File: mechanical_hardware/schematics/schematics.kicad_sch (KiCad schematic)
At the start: 19 parts, among them J1 Raspberry_Pi_4, J2 Encoder, J3 Encoder, M1 Motor_DC, M2 Motor_DC, SW1 PWR, U1 5.1V - Pi, U2 5V ESP32, U3 11.5V motors, U4 ESP32-C3, U5 MPU-9250

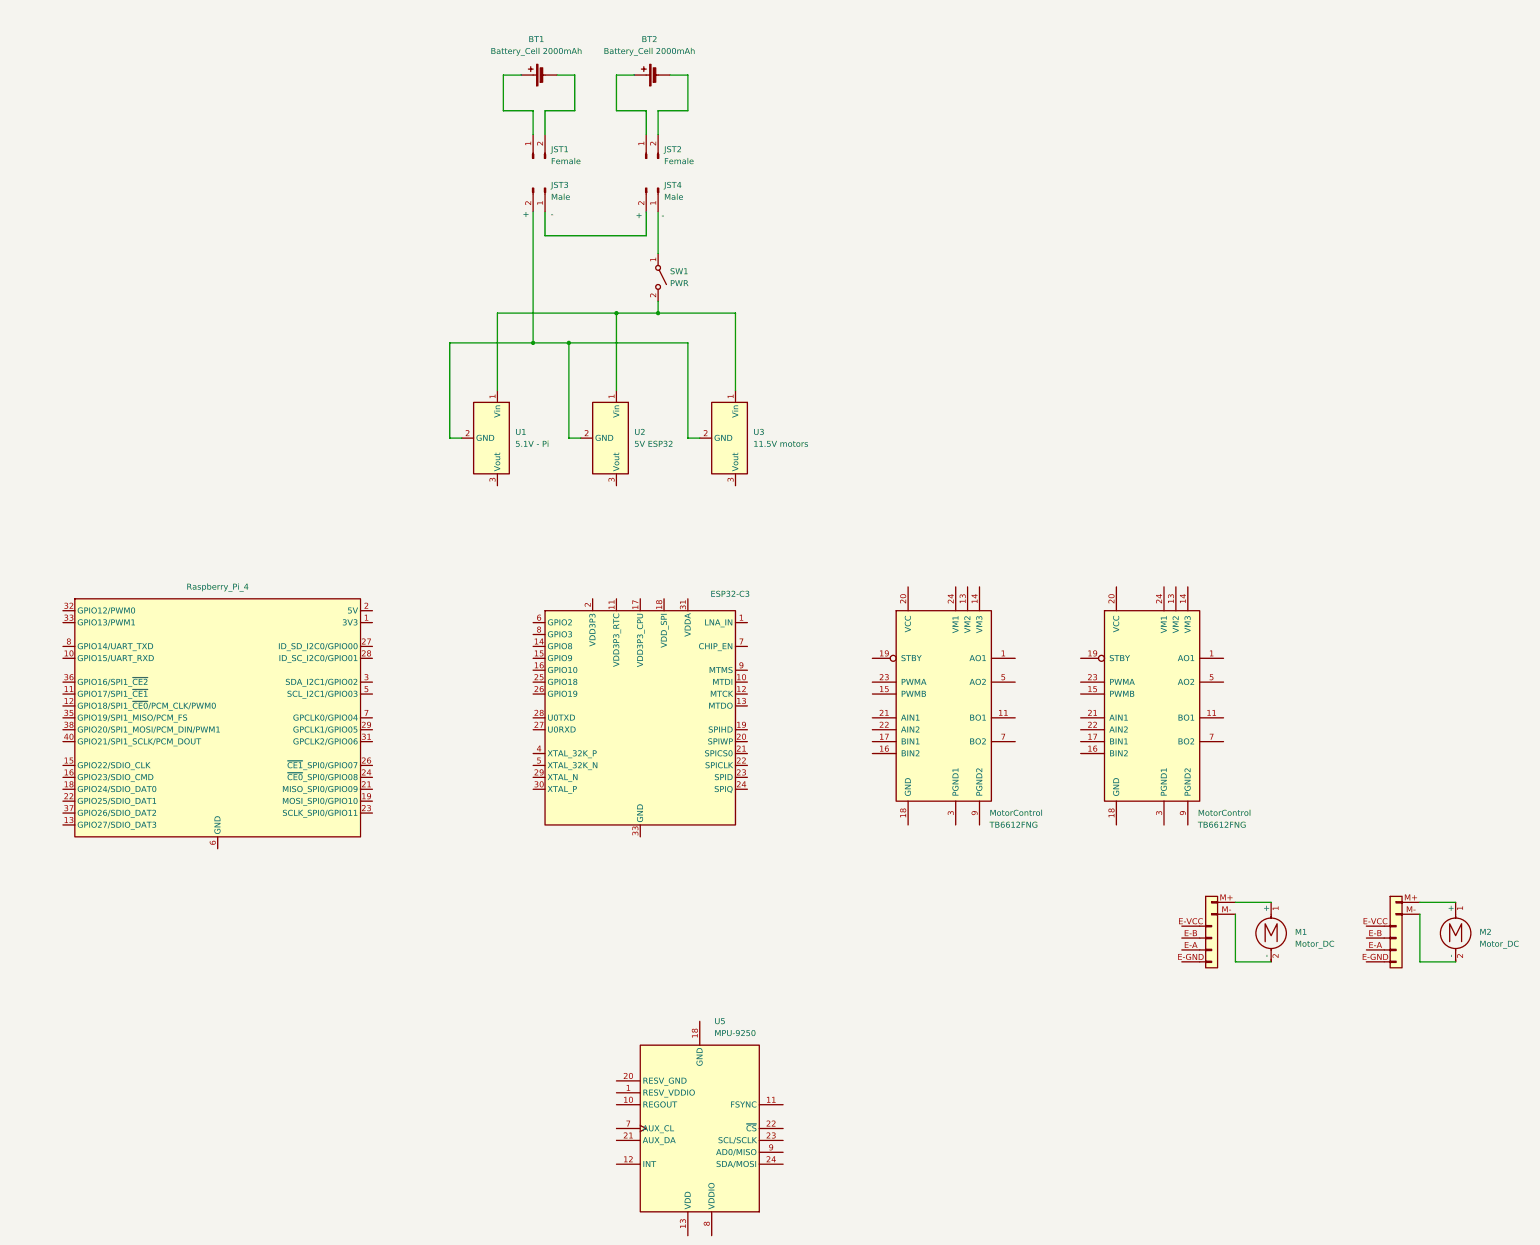
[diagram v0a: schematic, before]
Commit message: schematics
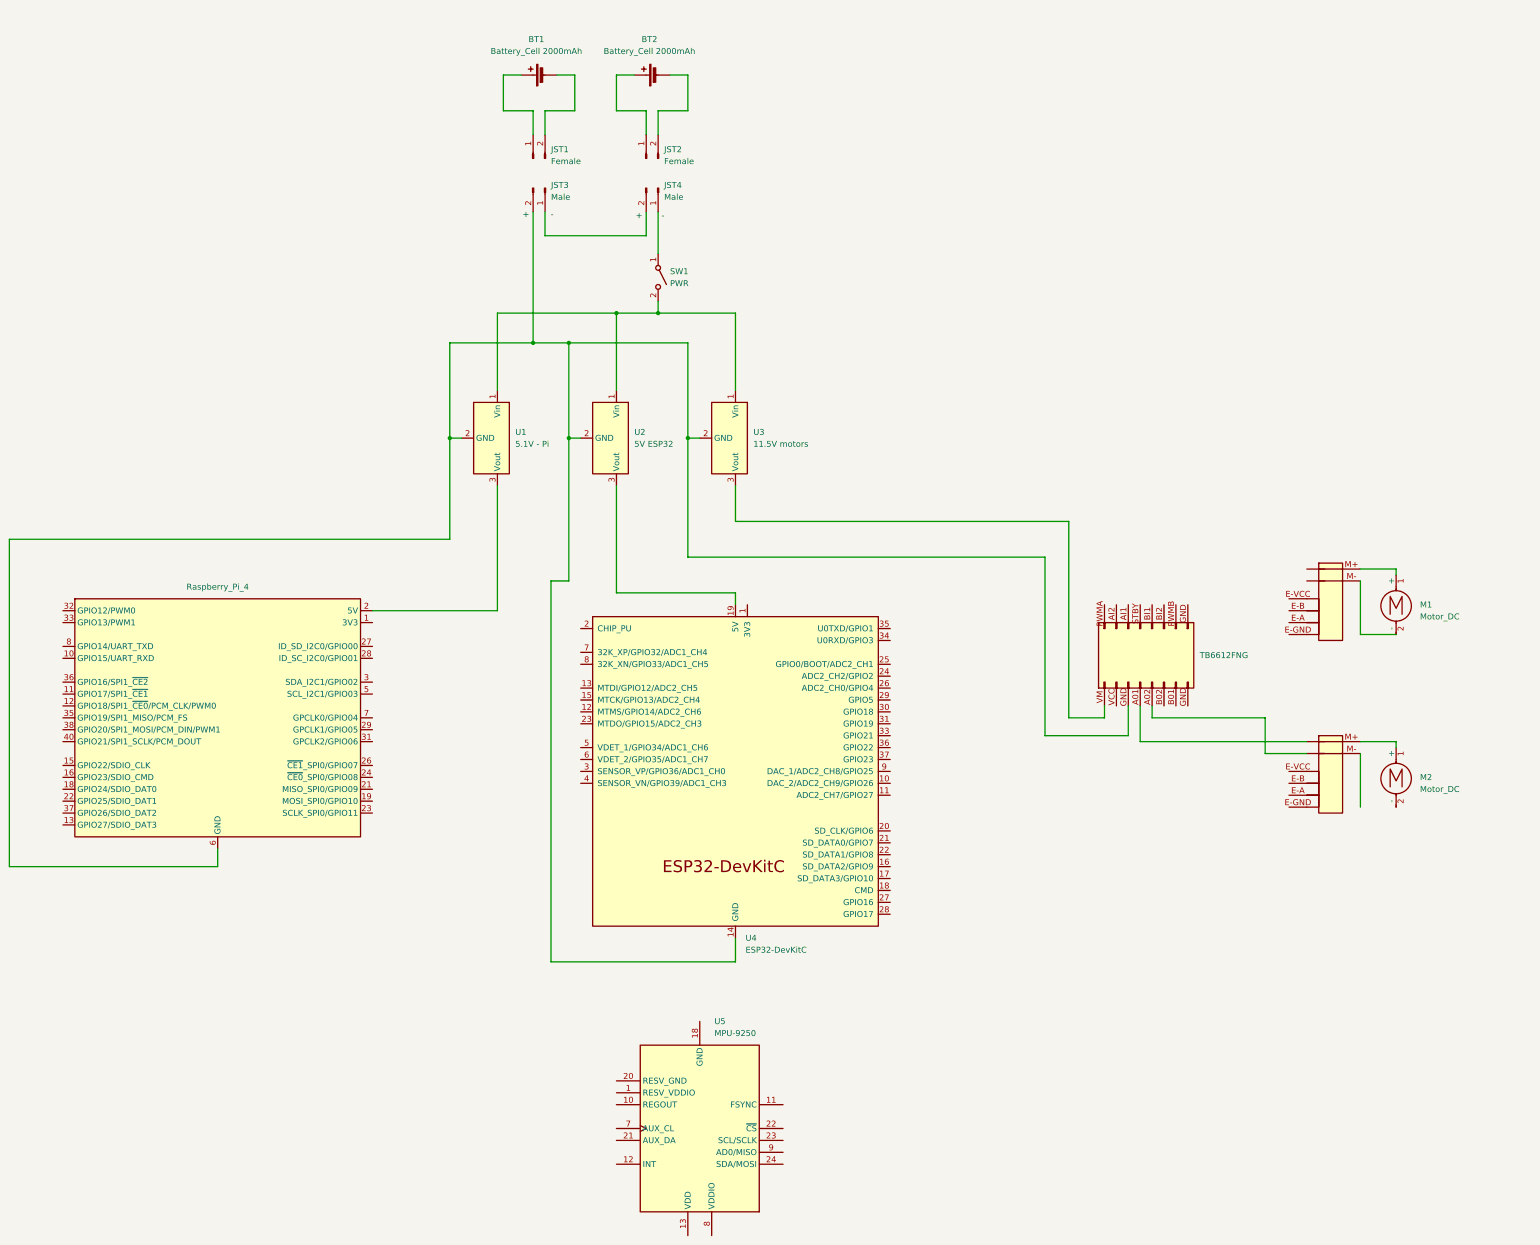
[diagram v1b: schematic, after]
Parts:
- removed J2, J3: Encoder, symbol Connector_Generic:Conn_01x06
- removed MotorControl (x2): TB6612FNG, Package_SO:SSOP-24_5.3x8.2mm_P0.65mm, symbol Driver_Motor:TB6612FNG
- removed U4: ESP32-C3, Package_DFN_QFN:QFN-32-1EP_5x5mm_P0.5mm_EP3.7x3.7mm, symbol MCU_Espressif:ESP32-C3
- added J4: TB6612FNG, symbol Connector_Generic:Conn_02x08_Top_Bottom
- added J5, J6: Encoder, symbol Connector_Generic:Conn_01x06
- added U4: ESP32-DevKitC, PCM_Espressif:ESP32-DevKitC, symbol PCM_Espressif:ESP32-DevKitC
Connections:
- net at M2.1 (+): now also J6.M+
- net at JST3.2 (Pin_2), U1.2 (GND), U2.2 (GND)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: now also J1.14 (GND), J1.20 (GND), J1.25 (GND), J1.30 (GND), J1.34 (GND), J1.39 (GND), J1.6 (GND), J1.9 (GND), J4.GND (Pin_16), U4.14 (GND), U4.32 (GND), U4.38 (GND)
- net at U1.3 (Vout): now also J1.2 (5V), J1.4 (5V)
- net at M1.1 (+): now also J5.M+
- net at M1.2 (-): now also J5.M-
- net at U2.3 (Vout): now also U4.19 (5V)
- net at U3.3 (Vout): now also J4.VM
- new net: J4.A01 (Pin_4), J6.
- new net: J4.A02 (Pin_5), J6.
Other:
- moved on the sheet: M1

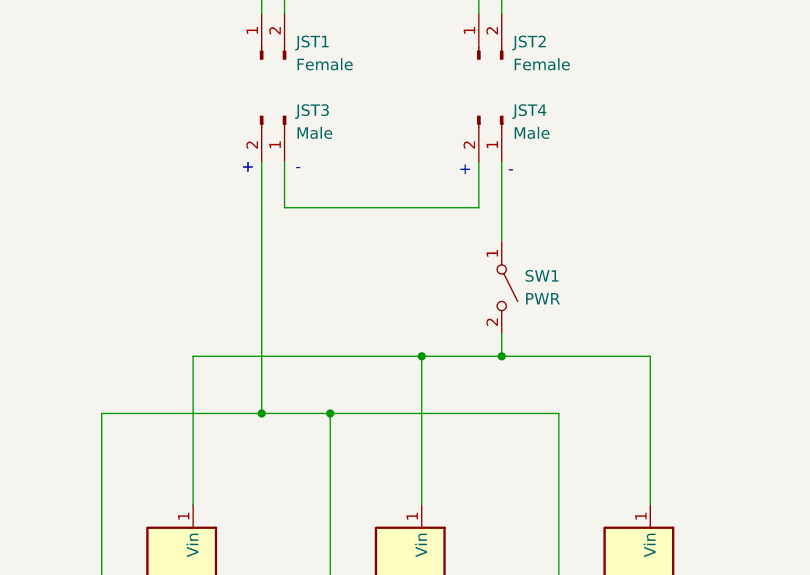
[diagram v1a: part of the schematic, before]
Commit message: fixed schematics
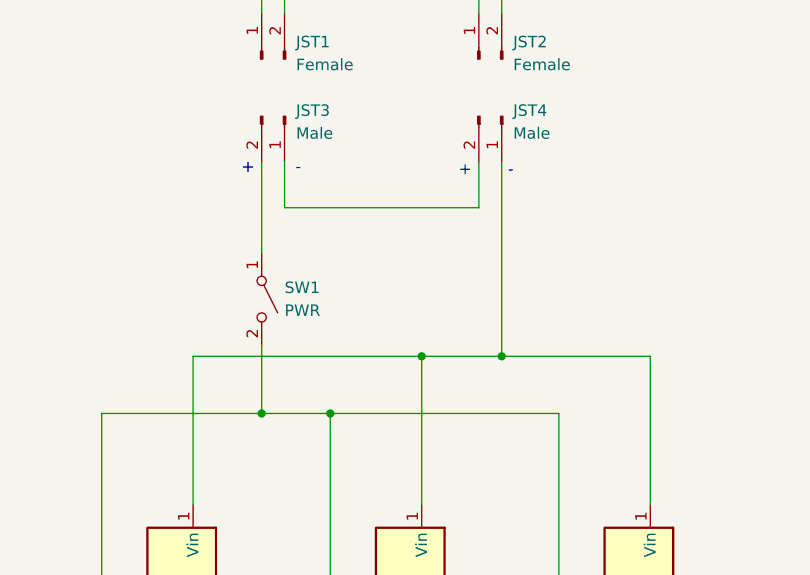
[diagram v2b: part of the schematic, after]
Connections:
- net at J4.GND (Pin_16): now also J1.14 (GND), J1.20 (GND), J1.25 (GND), J1.30 (GND), J1.34 (GND), J1.39 (GND), J1.6 (GND), J1.9 (GND), SW1.2 (B), U1.2 (GND), U2.2 (GND), U3.2 (GND), U4.14 (GND), U4.32 (GND), U4.38 (GND)
- net at SW1.1 (A): now also JST3.2 (Pin_2); no longer JST4.1 (Pin_1)
- net at U1.1 (Vin), U2.1 (Vin), U3.1 (Vin): now also JST4.1 (Pin_1); no longer SW1.2 (B)
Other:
- moved on the sheet: SW1
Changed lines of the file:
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@@
 	(wire
 		(pts
-			(xy 160.02 57.15) (xy 160.02 85.09)
+			(xy 160.02 57.15) (xy 160.02 67.31)
 		)
 		(stroke
@@
 	(wire
 		(pts
+			(xy 160.02 77.47) (xy 160.02 85.09)
+		)
+		(stroke
+			(width 0)
+			(type default)
+		)
+	)
+	(wire
+		(pts
 			(xy 336.55 170.18) (xy 344.17 170.18)
 		)
@@
 	(wire
 		(pts
-			(xy 186.69 76.2) (xy 186.69 78.74)
-		)
-		(stroke
-			(width 0)
-			(type default)
-		)
-	)
-	(wire
-		(pts
 			(xy 184.15 62.23) (xy 184.15 57.15)
 		)
@@
 	(wire
 		(pts
+			(xy 186.69 78.74) (xy 203.2 78.74)
+		)
+		(stroke
+			(width 0)
+			(type default)
+		)
+	)
+	(wire
+		(pts
 			(xy 316.23 165.1) (xy 316.23 172.72)
 		)
@@
 	(wire
 		(pts
+			(xy 186.69 57.15) (xy 186.69 78.74)
+		)
+		(stroke
+			(width 0)
+			(type default)
+		)
+	)
+	(wire
+		(pts
 			(xy 163.83 135.89) (xy 163.83 217.17)
 		)
@@
 	(wire
 		(pts
-			(xy 186.69 78.74) (xy 203.2 78.74)
-		)
-		(stroke
-			(width 0)
-			(type default)
-		)
-	)
-	(wire
-		(pts
 			(xy 153.67 27.94) (xy 153.67 35.56)
 		)
@@
 		(pts
 			(xy 186.69 35.56) (xy 186.69 40.64)
-		)
-		(stroke
-			(width 0)
-			(type default)
-		)
-	)
-	(wire
-		(pts
-			(xy 186.69 57.15) (xy 186.69 66.04)
 		)
 		(stroke
@@
 	(symbol
 		(lib_id "Switch:SW_SPST")
-		(at 186.69 71.12 270)
+		(at 160.02 72.39 270)
 		(unit 1)
 		(body_style 1)
@@
 		(fields_autoplaced yes)
 		(property "Reference" "SW1"
-			(at 189.23 69.8499 90)
+			(at 162.56 71.1199 90)
 			(show_name no)
 			(do_not_autoplace no)
@@
 		)
 		(property "Value" "PWR"
-			(at 189.23 72.3899 90)
+			(at 162.56 73.6599 90)
 			(show_name no)
 			(do_not_autoplace no)
@@
 		)
 		(property "Footprint" ""
-			(at 186.69 71.12 0)
+			(at 160.02 72.39 0)
 			(hide yes)
 			(show_name no)
@@
 		)
 		(property "Datasheet" ""
-			(at 186.69 71.12 0)
+			(at 160.02 72.39 0)
 			(hide yes)
 			(show_name no)
@@
 		)
 		(property "Description" "Single Pole Single Throw (SPST) switch"
-			(at 186.69 71.12 0)
-			(hide yes)
-			(show_name no)
+			(at 160.02 72.39 0)
+			(hide yes)
+			(show_name no)

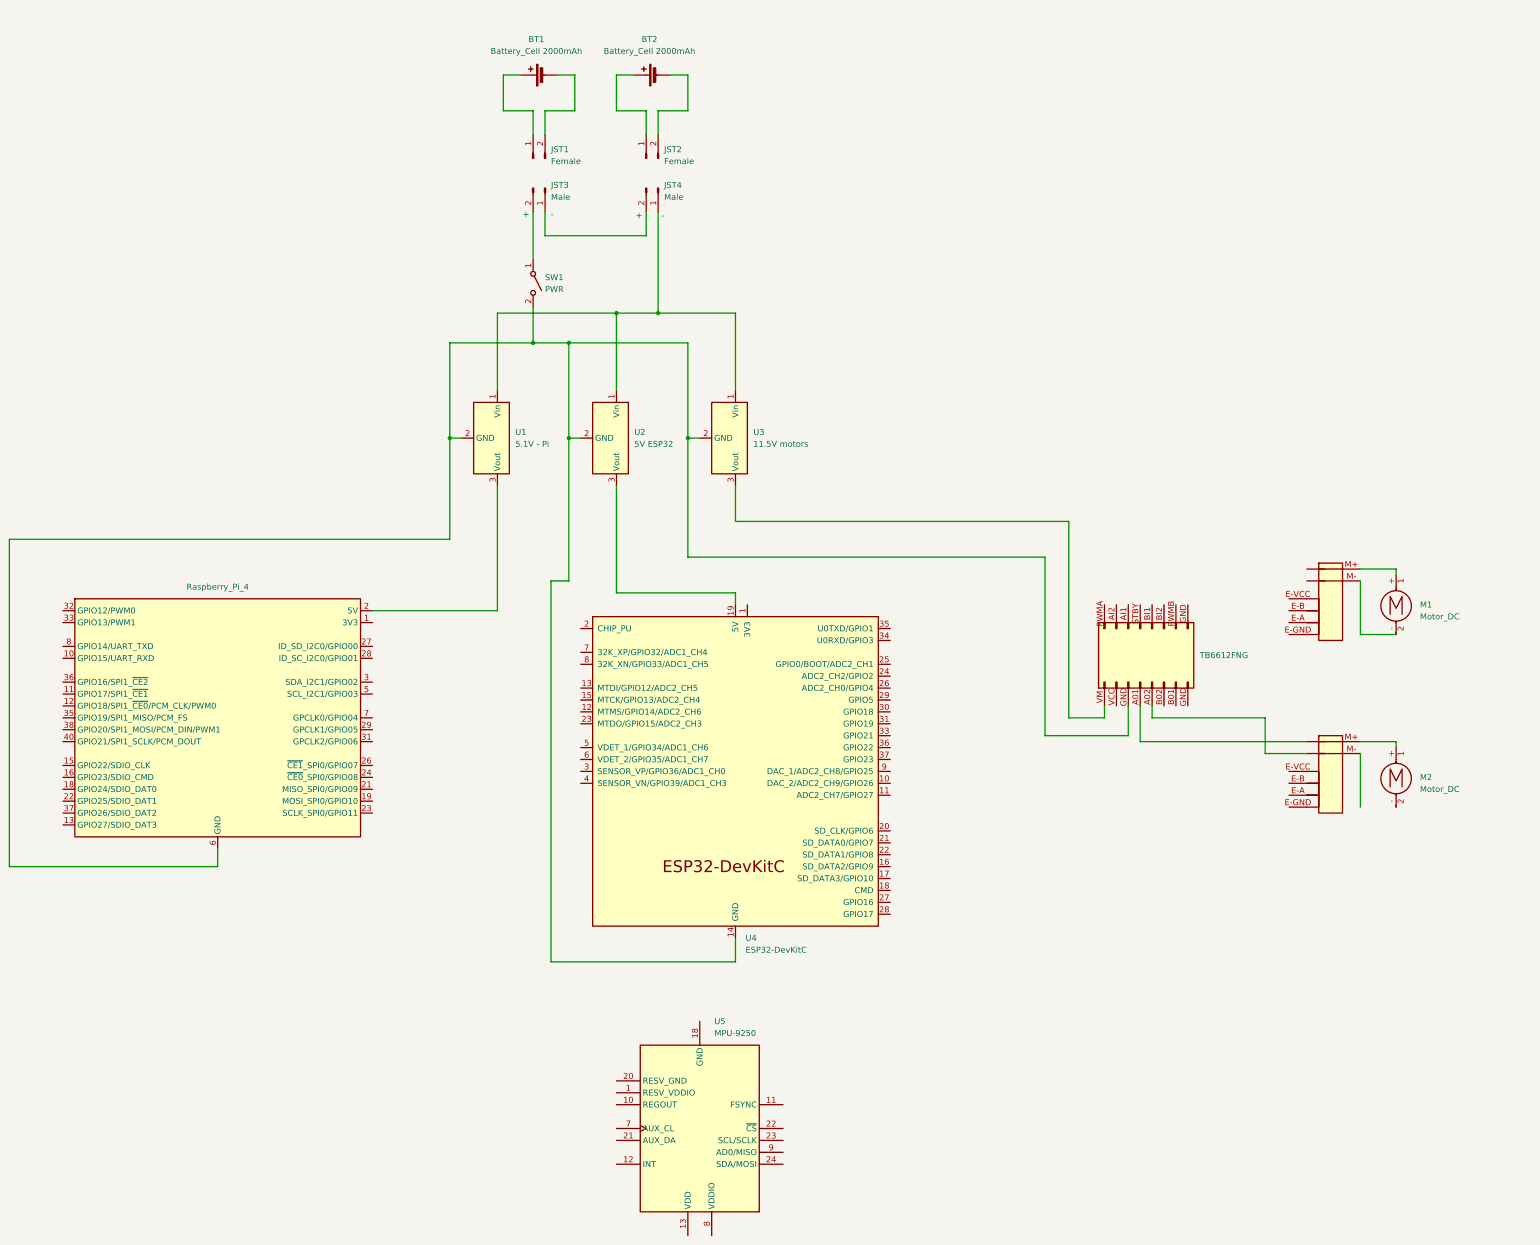
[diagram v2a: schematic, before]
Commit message: schematics
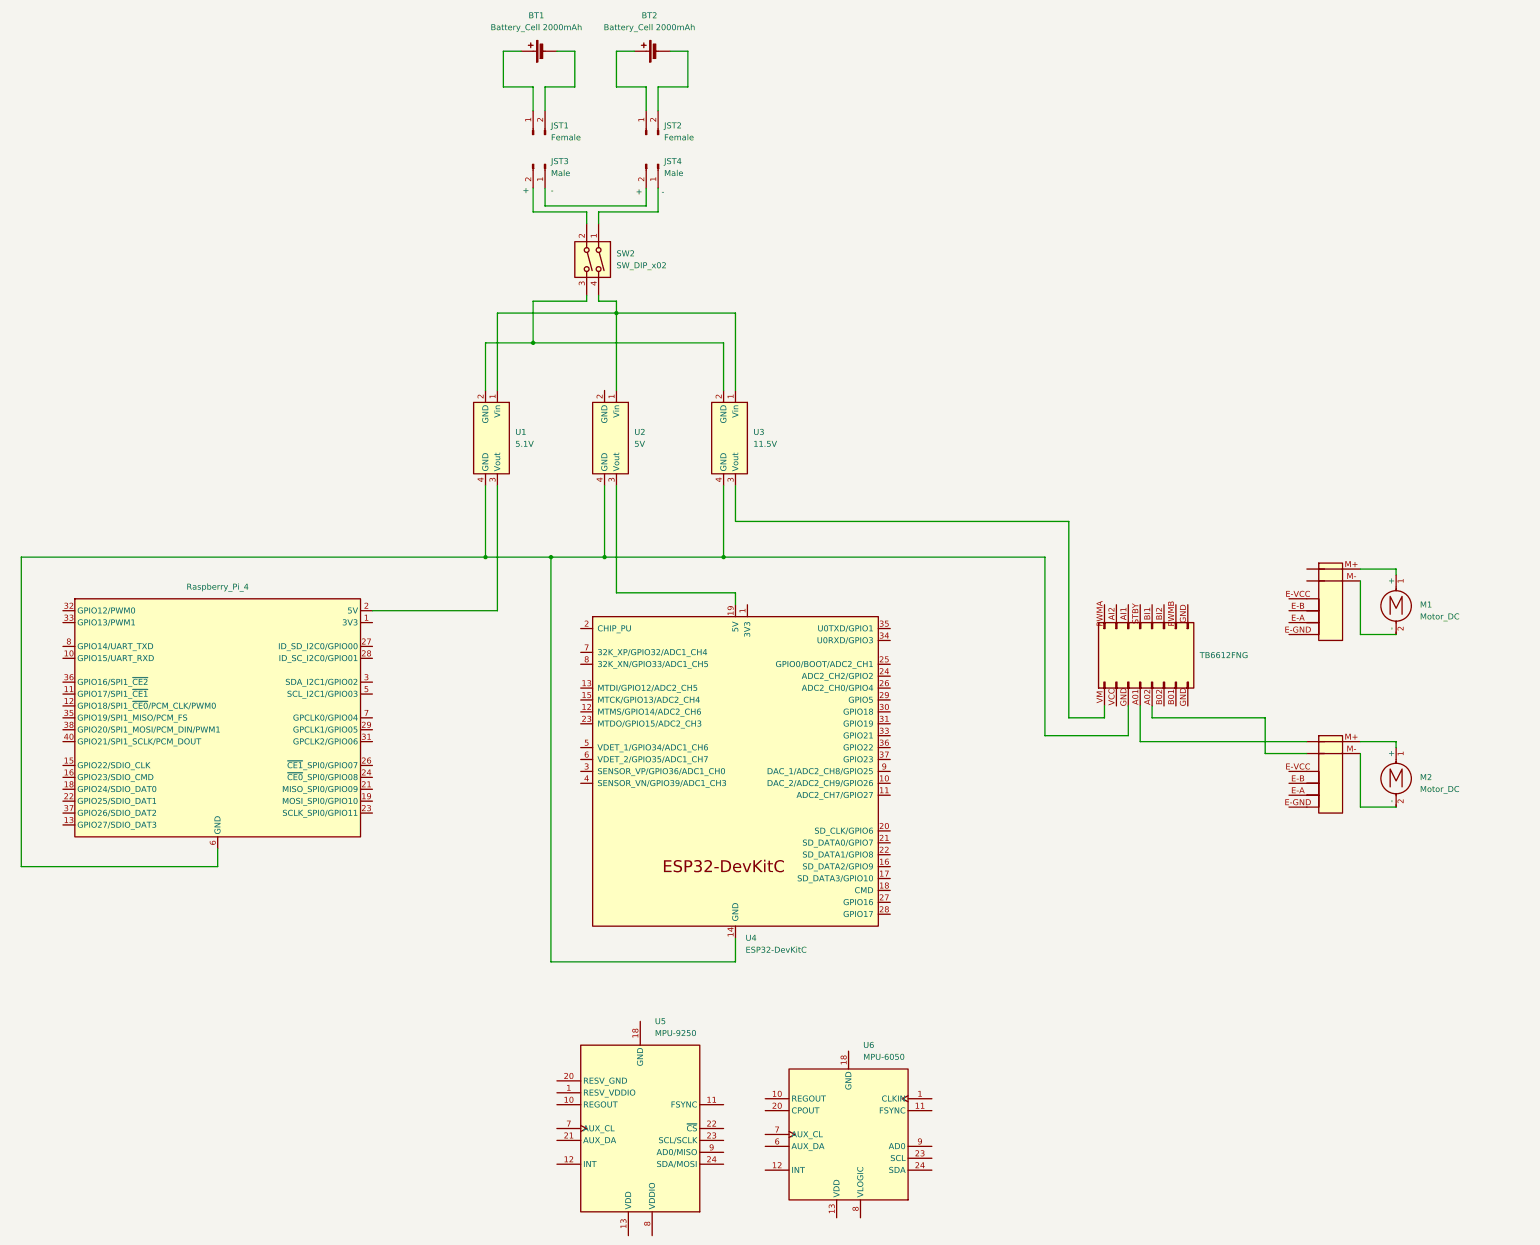
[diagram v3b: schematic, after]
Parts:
- removed SW1: PWR, symbol Switch:SW_SPST
- added SW2: SW_DIP_x02, symbol Switch:SW_DIP_x02
- added U6: MPU-6050, Sensor_Motion:InvenSense_QFN-24_4x4mm_P0.5mm, symbol Sensor_Motion:MPU-6050
- U1: value 5.1V - Pi -> 5.1V
- U2: value 5V ESP32 -> 5V
- U3: value 11.5V motors -> 11.5V
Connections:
- net at J1.14 (GND), J1.20 (GND), J1.25 (GND)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: now also U1.4 (GND), U2.4 (GND), U3.4 (GND); no longer U1.2 (GND), U2.2 (GND), U3.2 (GND)
- net at JST3.2 (Pin_2): now also SW2.2
- net at U1.1 (Vin), U2.1 (Vin), U3.1 (Vin): now also SW2.4; no longer JST4.1 (Pin_1)
- net at J6.M-: now also M2.2 (-)
- new net: SW2.3, U1.2 (GND), U3.2 (GND)
- new net: JST4.1 (Pin_1), SW2.1
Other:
- moved on the sheet: BT1, BT2, JST1, JST2, JST3, JST4, U5
